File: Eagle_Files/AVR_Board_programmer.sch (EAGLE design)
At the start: 20 parts, among them J1 10118192-0001LF, U1 CP2102N-A01-GQFN20

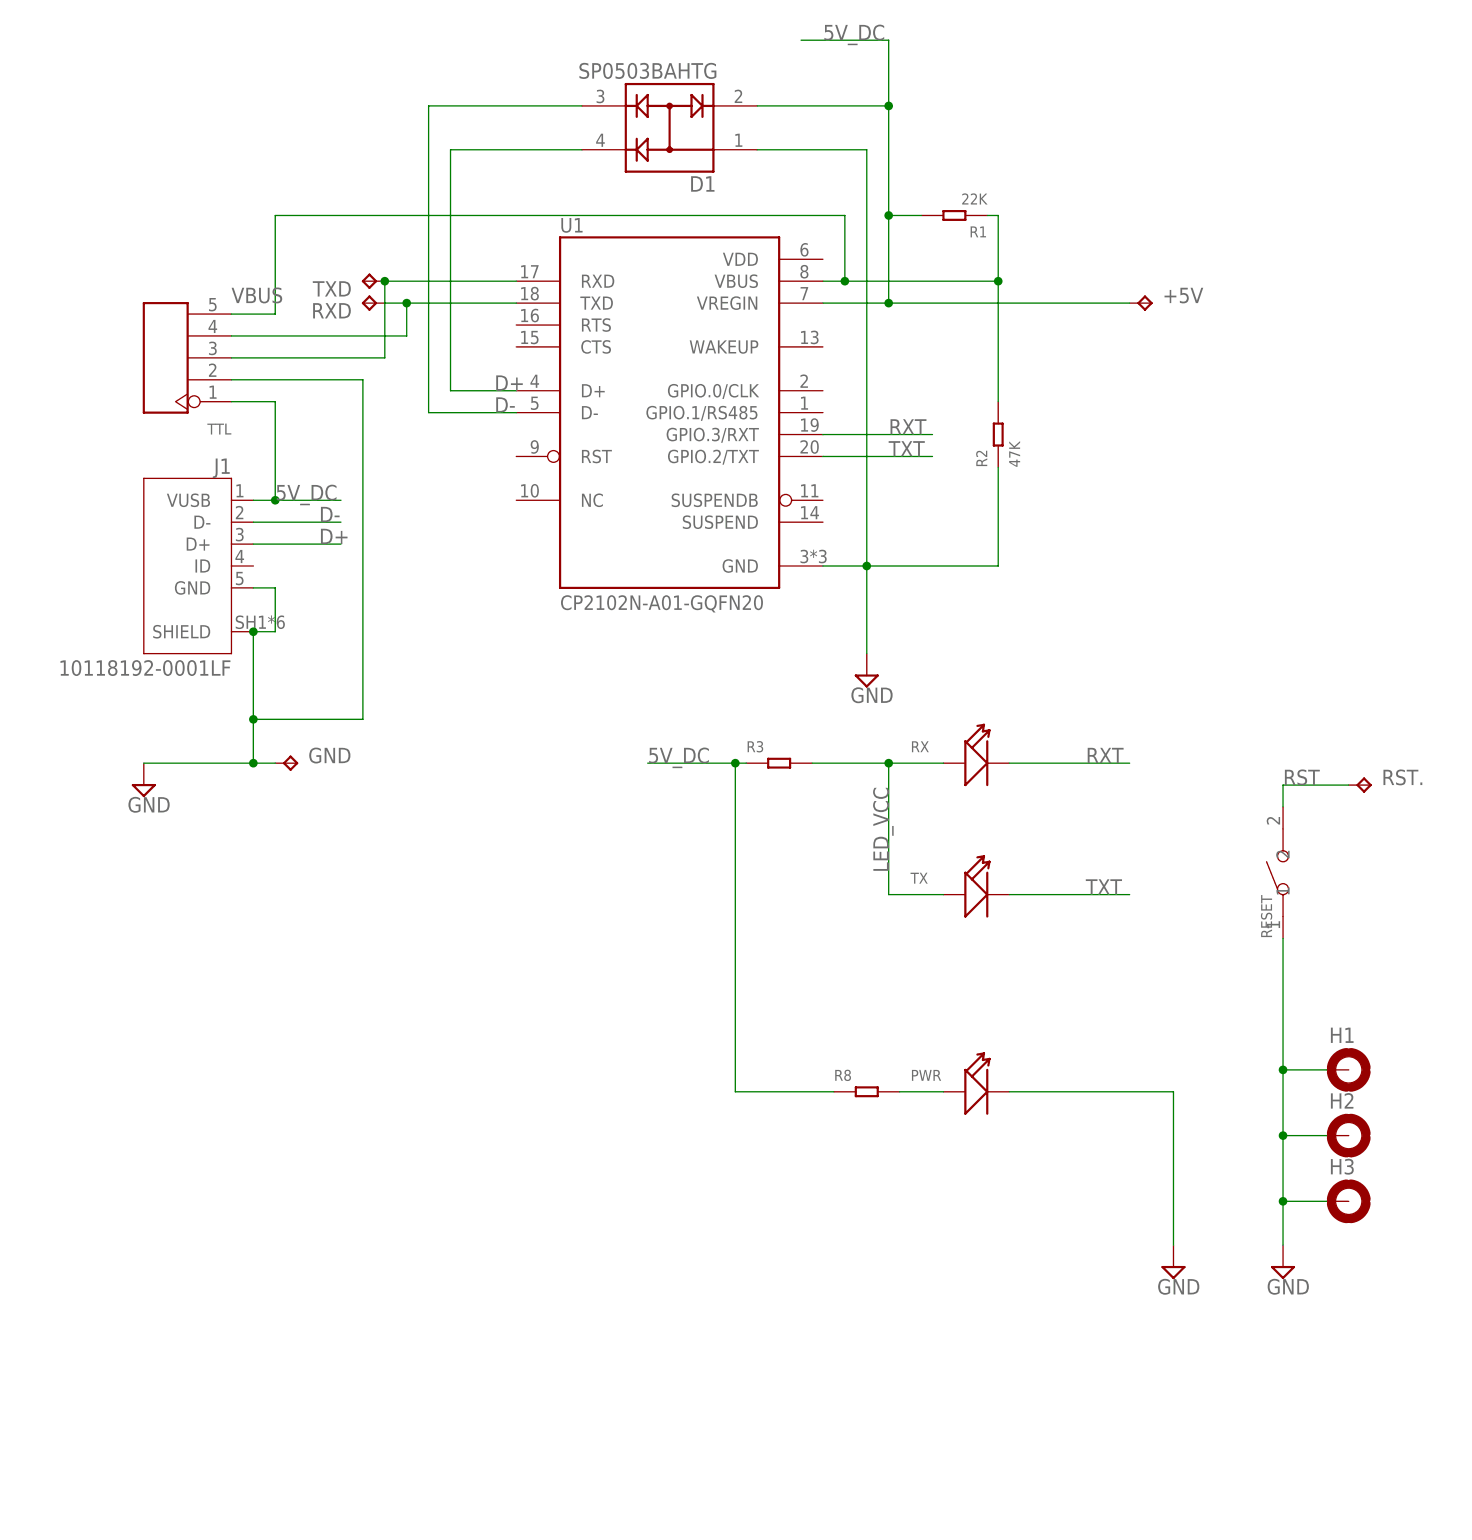
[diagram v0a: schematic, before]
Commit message: pulled latest fixes from master
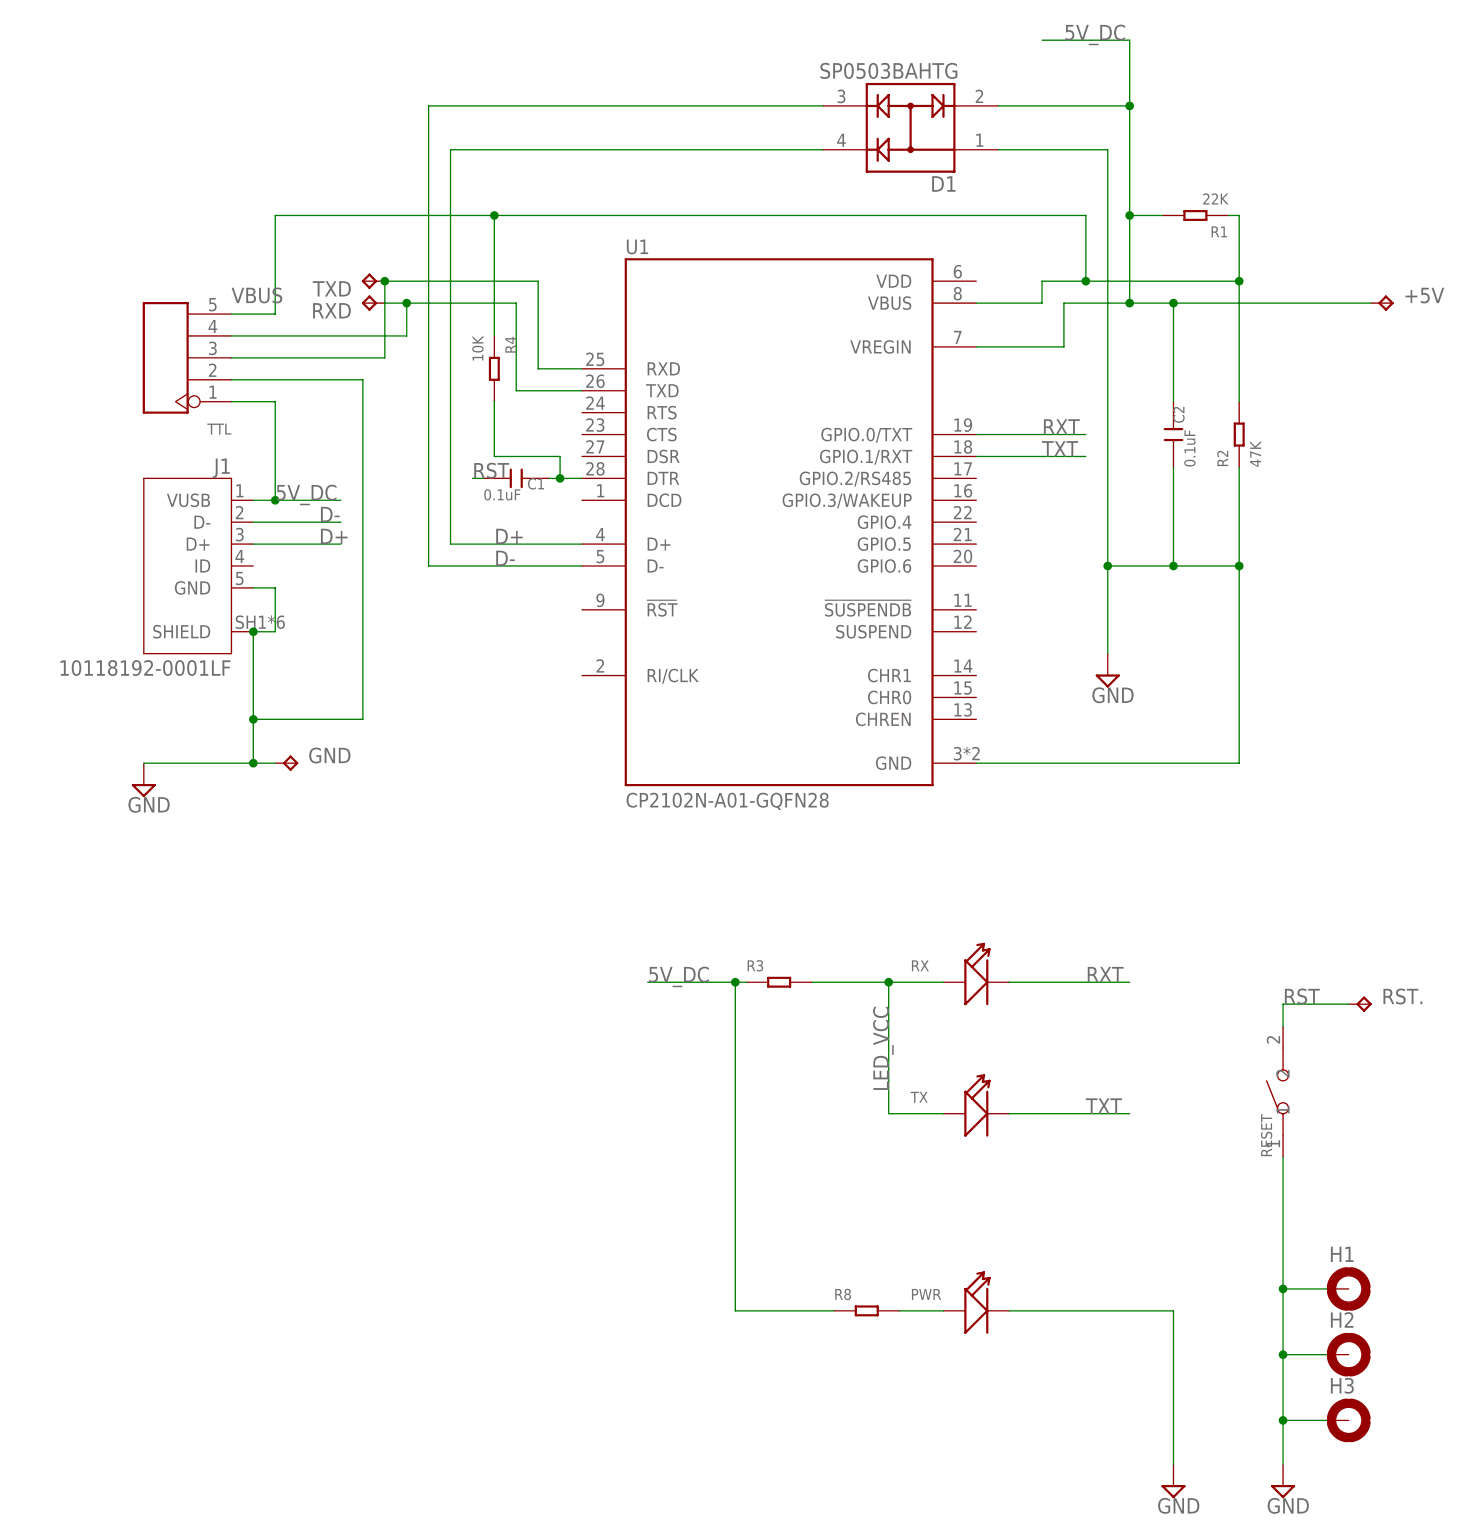
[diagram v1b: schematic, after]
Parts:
- added C1, C2: 0.1uF, PiezoFFC:CERAMIC-1NF-50V-10%-X7R(0402)CAP_0402
- added R4: 10K, PiezoFFC:SMD-RES-0R-5%-1/16W(0402)
- U1: value CP2102N-A01-GQFN20 -> CP2102N-A01-GQFN28; device PiezoFFC:CP2102N-A01-GQFN20 -> PiezoFFC:CP2102N-A01-GQFN28
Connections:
- new net PGM_RST: C1.2, R4.2, U1.DTR
- net 5V_DC: now also C2.2
- net GND: now also C2.1
- net RST: now also C1.1
- net RXT: now also U1.GPIO.0/TXT; no longer U1.GPIO.3/RXT
- net TXT: now also U1.GPIO.1/RXT; no longer U1.GPIO.2/TXT
- net VBUS: now also R4.1
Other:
- moved on the sheet: +5V, D1, H1, H2, H3, PWR, R1, R2, R3, R8, RESET, RST.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
